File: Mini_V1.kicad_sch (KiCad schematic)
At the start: 31 parts, among them J1 PJ-035DH, J2 Conn_01x05, J3 Conn_01x01_Pin, SW1 SW_Rotary_1x3_MP, SW2 SW_Push_DPDT, U1 LM2596S-5, U2 LM2596S-ADJ, U3 NE555P, U4 L7809

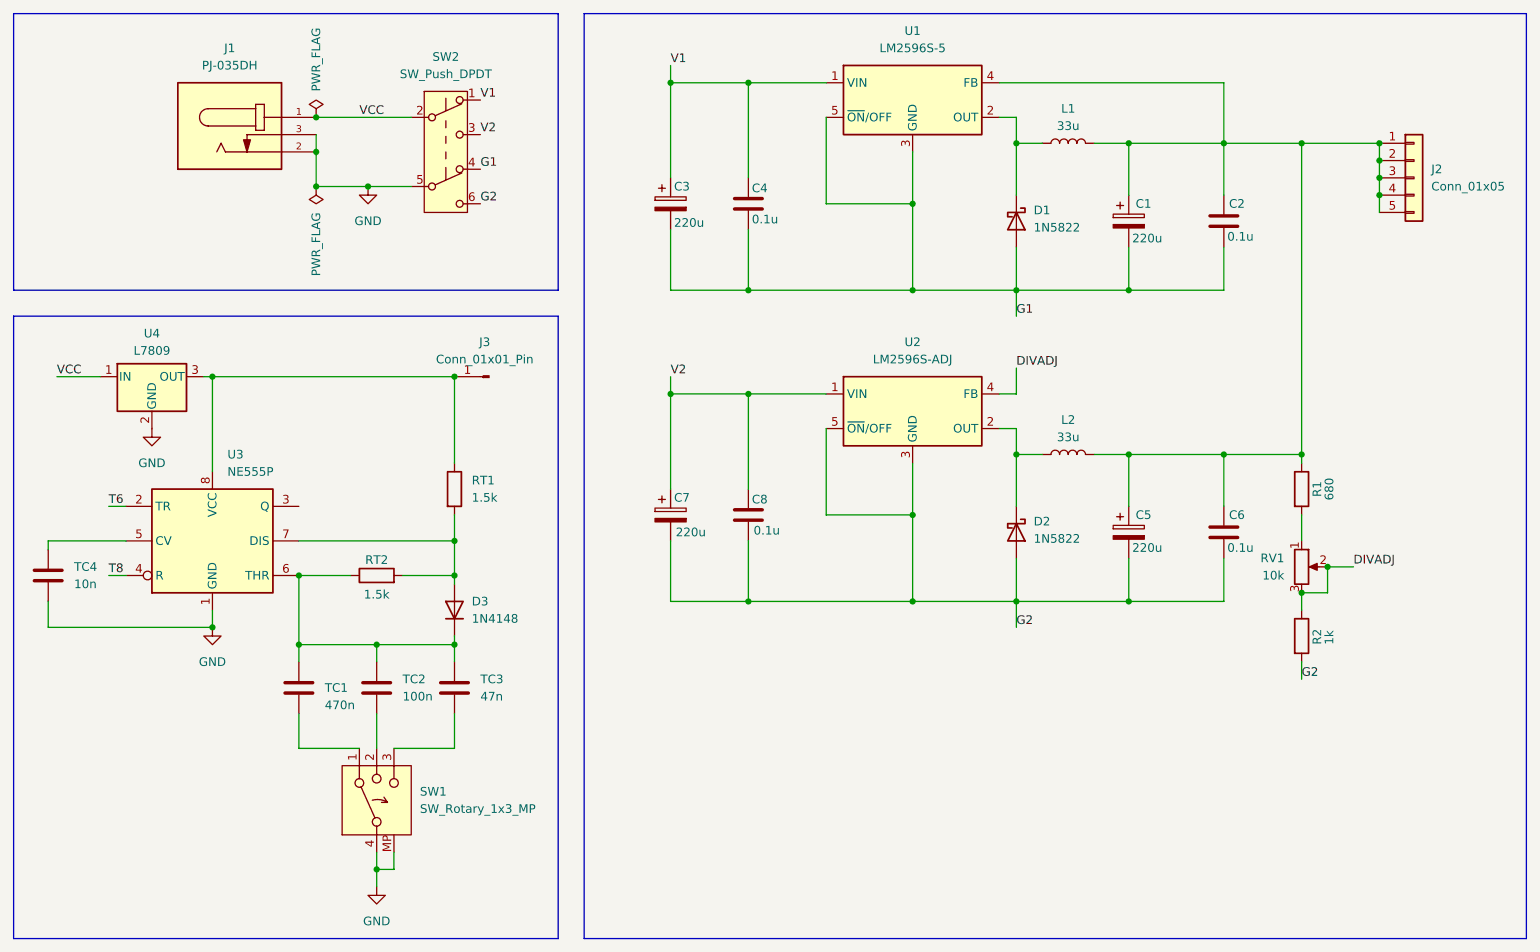
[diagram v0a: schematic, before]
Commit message: Add files via upload
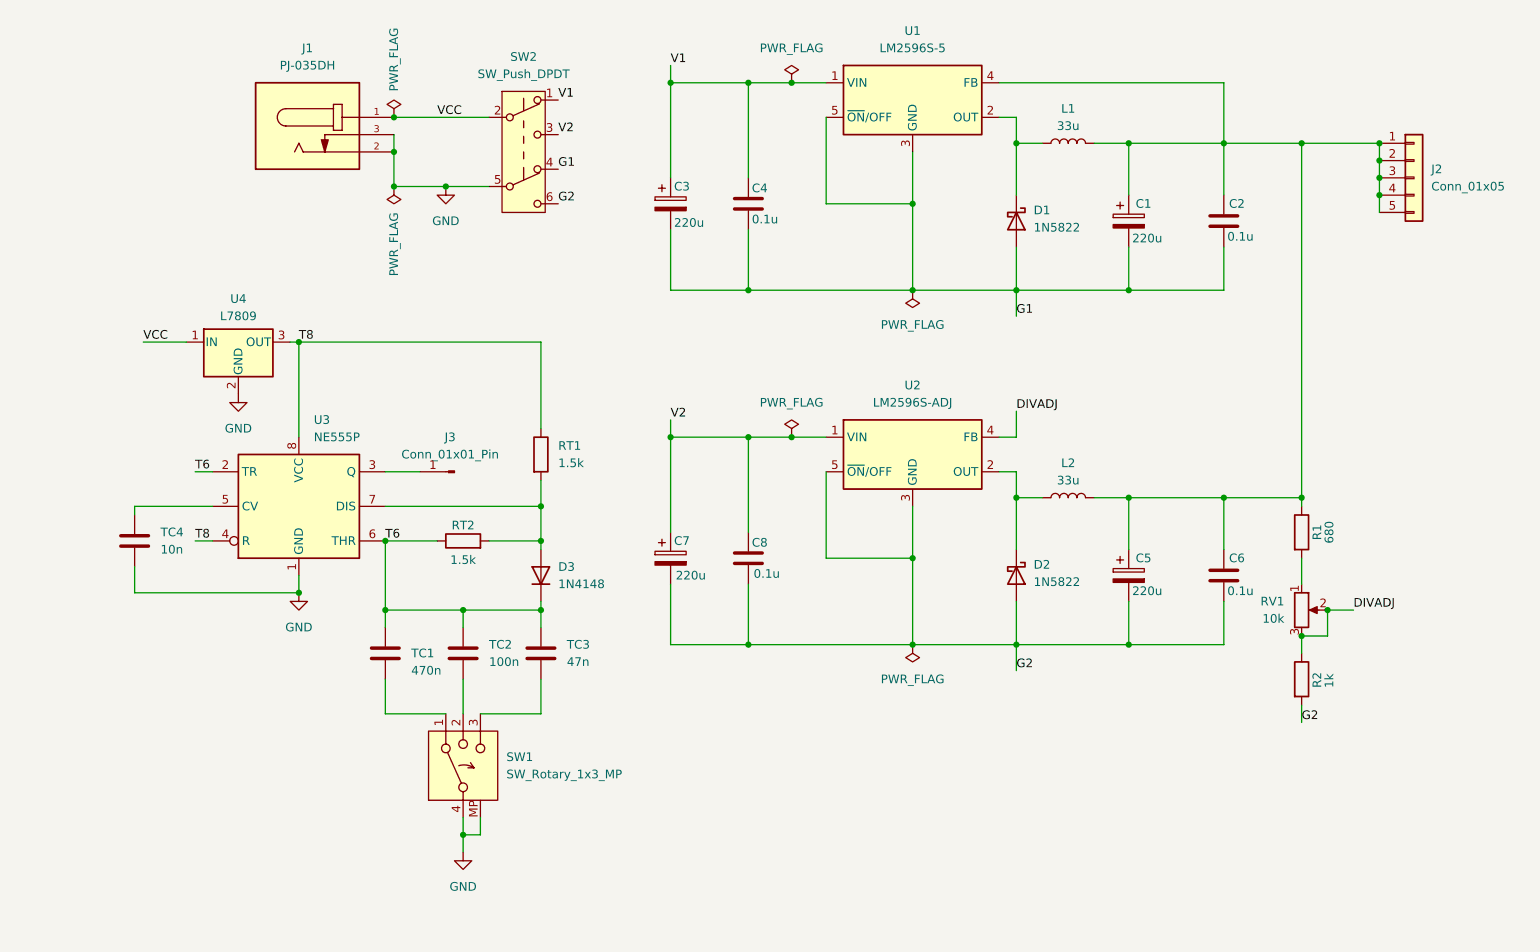
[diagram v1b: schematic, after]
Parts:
- C2, C4, C6, C8, TC1, TC2, TC3, TC4: footprint (none) -> Capacitor_SMD:C_0805_2012Metric_Pad1.18x1.45mm_HandSolder
- D3: footprint (none) -> Diode_THT:D_DO-35_SOD27_P7.62mm_Horizontal
- J3: footprint (none) -> Connector_PinHeader_2.00mm:PinHeader_1x01_P2.00mm_Vertical
- RT1, RT2: footprint (none) -> Resistor_SMD:R_0805_2012Metric_Pad1.20x1.40mm_HandSolder
- RV1: footprint (none) -> Potentiometer_THT:Potentiometer_Piher_PC-16_Single_Horizontal
- SW1: footprint (none) -> Rotary_Encoder:RotaryEncoder_Bourns_Vertical_PEC12R-3x17F-Nxxxx(custom)
- SW2: footprint (none) -> TL2230OAF140:SW_TL2230OAF140
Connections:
- net T6: now also D3.1 (K), RT2.1, TC1.1, TC2.1, TC3.1, U3.6 (THR)
- net T8: now also RT1.1, U3.8 (VCC), U4.3 (OUT)
- net at U3.3 (Q): now also J3.1 (Pin_1)
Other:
- moved on the sheet: C5, C6, C7, C8, D2, D3, J1, J3, L2, R1, R2, RT1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
